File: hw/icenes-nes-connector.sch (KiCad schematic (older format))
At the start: 5 parts

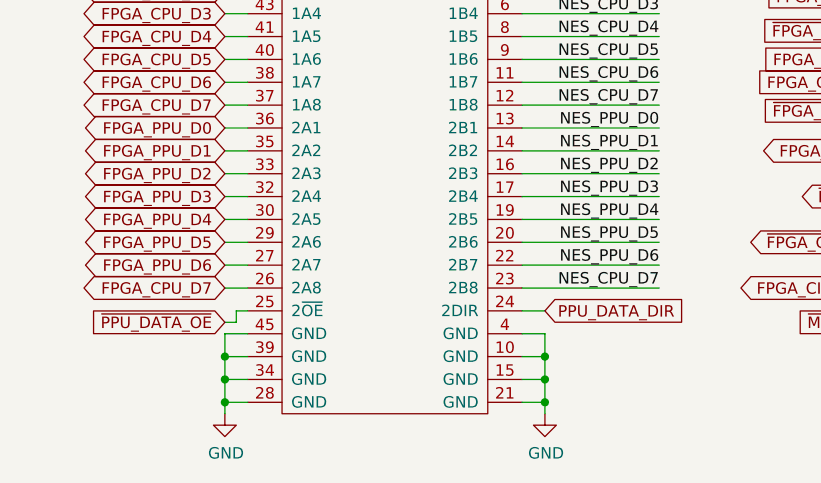
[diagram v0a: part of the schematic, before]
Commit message: .
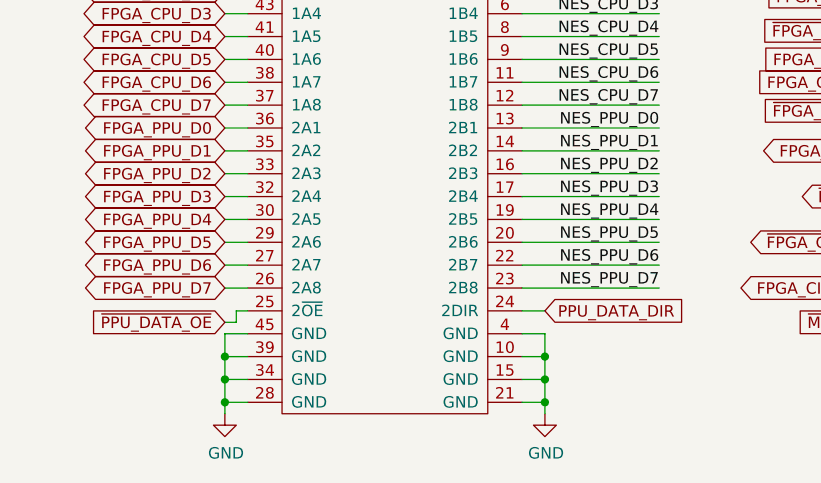
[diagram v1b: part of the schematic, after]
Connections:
- net FPGA_CPU_D7: no longer U?.26 (2A8)
- net NES_CPU_D7: no longer U?.23 (2B8)
- net NES_PPU_D7: now also U?.23 (2B8)
- new net FPGA_PPU_D7: U?.26 (2A8)
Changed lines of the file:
@@
 FPGA_PPU_D6
 Text GLabel 1550 5800 0    50   BiDi ~ 0
-FPGA_CPU_D7
+FPGA_PPU_D7
 Text GLabel 1550 5950 0    50   Input ~ 0
 ~PPU_DATA_OE
@@
 	2850 5700 3450 5700
 Text Label 3450 5800 2    50   ~ 0
-NES_CPU_D7
+NES_PPU_D7
 Wire Wire Line
 	2850 5800 3450 5800
